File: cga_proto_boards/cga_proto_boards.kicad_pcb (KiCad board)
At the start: 2 copper layers, 58.7 x 27 mm, 19 parts, among them Q1 2N7002, T1 TRRS, U1 Elite-C

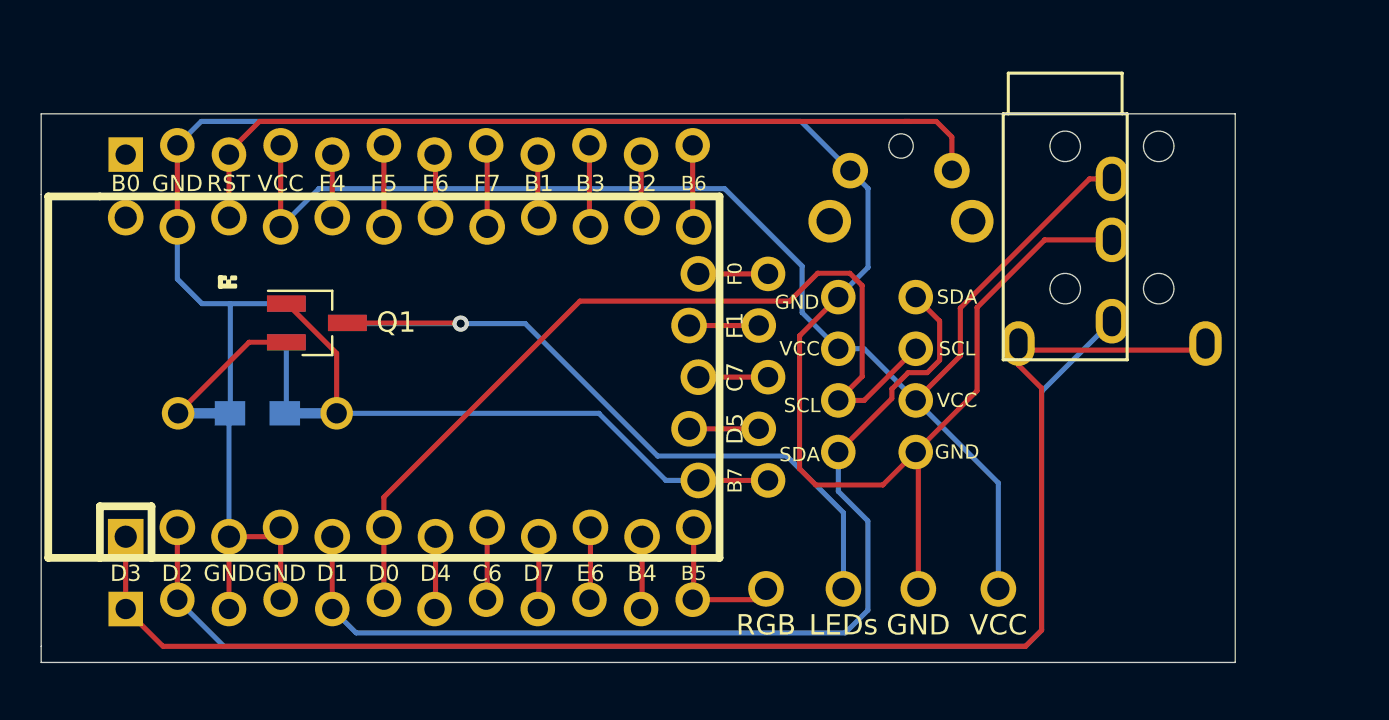
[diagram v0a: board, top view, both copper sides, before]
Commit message: Finalize v1 of the sideways cga proto board
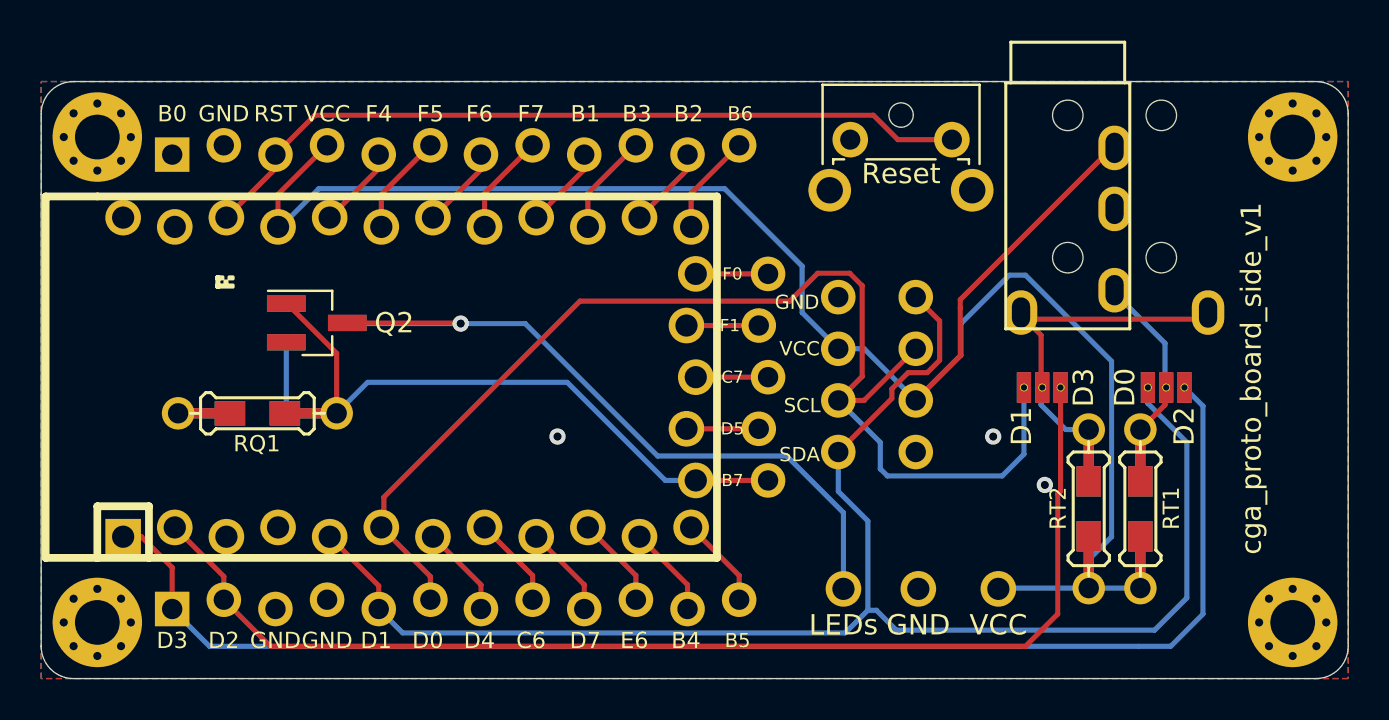
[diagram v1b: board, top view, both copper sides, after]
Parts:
- removed the ? at (73.9, 49.1)
- removed the ? at (69.2, 44.1)
- removed the ? at (3.68, 5.59)
- removed the ? at (61.6, 44.2)
- removed H4: VCC, Keebio-Parts:SinglePad
- removed the Q1 at (39.8, 29.3)
- added ?: , , F.Cu at (-15.9, 34.9)
- added ?: , , F.Cu at (82.4, 14.7)
- added ?: , , F.Cu at (-9.40, 31.4)
- added J1: 3_way_jumper, Keebio-Parts:3_way_solder_jumper, F.Cu at (75.0, 32.5)
- added J2: 3_way_jumper, Keebio-Parts:3_way_solder_jumper, F.Cu at (81.1, 32.5)
- added Q2: 2N7002, Keebio-Parts:SOT-23_Handsoldering, F.Cu at (39.8, 29.3)
- added RT1: 4.7k, Keebio-Parts:Resistor-2-sided, F.Cu at (80.3, 38.5)
- added RT2: 4.7k, Keebio-Parts:Resistor-2-sided, F.Cu at (77.7, 38.5)
- added Screw1: MountingHole_2.2mm_M2_Pad_Via, MountingHole:MountingHole_2.2mm_M2_Pad_Via, F.Cu at (29.0, 20.2)
- added Screw2: MountingHole_2.2mm_M2_Pad_Via, MountingHole:MountingHole_2.2mm_M2_Pad_Via, F.Cu at (87.8, 20.2)
- added Screw3: MountingHole_2.2mm_M2_Pad_Via, MountingHole:MountingHole_2.2mm_M2_Pad_Via, F.Cu at (87.8, 44.1)
- added Screw4: MountingHole_2.2mm_M2_Pad_Via, MountingHole:MountingHole_2.2mm_M2_Pad_Via, F.Cu at (29.0, 44.1)
- H2: value RGB -> GND
- H3: value GND -> VCC
- RQ1: footprint Keebio-Parts:Resistor-Hybrid-Back -> Keebio-Parts:Resistor-2-sided
- Reset: footprint Keebio-Parts:SW_Tactile_SPST_Angled_MJTP1117 -> Keebio-Parts:SW_Two_sided
- moved H2 7.49 mm to (69.3, 42.4)
- moved H3 3.94 mm to (73.3, 42.4)
- moved Cs1 2.29 mm to (32.6, 43.2)
- moved Cs2 2.29 mm to (32.6, 20.8)
- moved T1 1.53 mm to (79.0, 17.5)
- moved Reset 1.52 mm to (71.0, 20.3)
- moved U1 0.13 mm to (44.2, 32.0)
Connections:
- Cs1 pad 1: TRRS1 -> TX
- Cs1 pad 2: TRRS2 -> RX
- H2 pad 1: RGB -> GND
- H3 pad 1: GND -> VCC
- U1 pad 1: TRRS1 -> TX
- U1 pad 2: TRRS2 -> RX
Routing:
- net GND: track 121.4 -> 1.05 mm, vias 0 -> 3
- net TX: track 0.00 -> 68.8 mm
- net RX: track 0.00 -> 58.5 mm
- net TRRS1: track 73.7 -> 17.8 mm
- net TRRS2: track 64.0 -> 8.44 mm
- net SDA: track 50.0 -> 76.8 mm
- net VCC: track 68.2 -> 91.2 mm
- net SCL: track 44.4 -> 61.0 mm
- net RESET: track 41.6 -> 38.7 mm
- net RGB: track 7.40 -> 4.53 mm
- net LEDs: track 32.7 -> 33.9 mm
- net col1: track 4.01 -> 5.08 mm
- net col7: track 4.03 -> 5.06 mm
- net col5: track 4.03 -> 5.06 mm
- net col4: track 3.12 -> 4.15 mm
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- added copper zone on B.Cu, net GND
- added copper zone on F.Cu, net GND
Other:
- board size 58.7 x 27 mm -> 64.3 x 29.4 mm
- board text added: "D0"
- board text added: "D1"
- board text added: "D2"
- board text added: "D3"
- board text added: "cga_proto_board_side_v1"
